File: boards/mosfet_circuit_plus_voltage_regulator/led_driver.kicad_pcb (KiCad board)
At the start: 2 copper layers, 75 x 50 mm, 26 parts, among them J1 Vin, J2 LED, J3 control_in, Q1 IRF4905 P-chan, Q2 BUZ11 N-chan, U1 MC34063AP

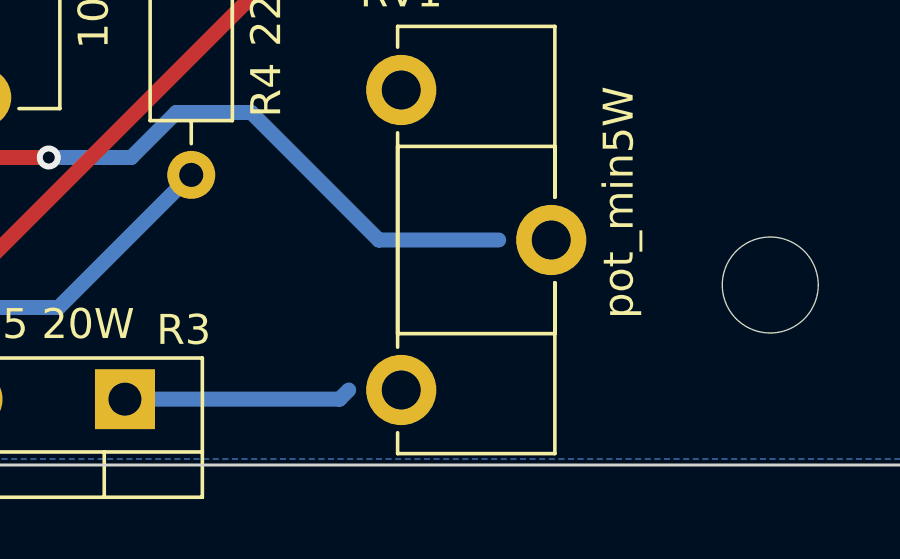
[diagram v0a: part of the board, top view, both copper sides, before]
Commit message: update gerbers
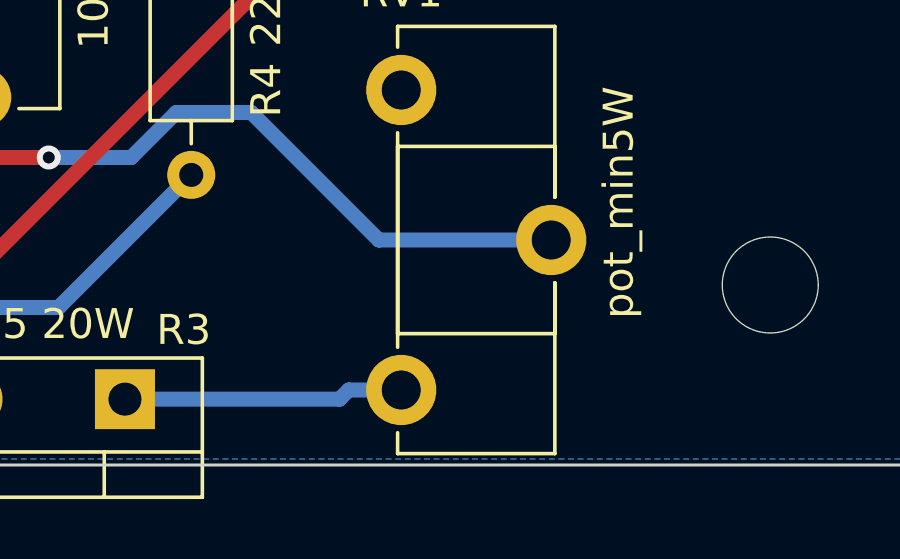
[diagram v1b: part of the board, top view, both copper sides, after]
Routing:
- net Net-(R3-Pad1): track 7.59 -> 9.34 mm
- net Net-(J2-Pad1): track 62.0 -> 63.7 mm
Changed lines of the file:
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@@
   (segment (start 94.485 79.235) (end 108 92.75) (width 0.5) (layer "F.Cu") (net 2))
   (via (at 131.75 92.75) (size 0.8) (drill 0.4) (layers "F.Cu" "B.Cu") (net 2))
-  (segment (start 142.75 95.5) (end 146.75 95.5) (width 0.5) (layer "B.Cu") (net 2))
+  (segment (start 142.75 95.5) (end 148.5 95.5) (width 0.5) (layer "B.Cu") (net 2))
+  (segment (start 136 91.25) (end 138.5 91.25) (width 0.5) (layer "B.Cu") (net 2))
+  (segment (start 131.75 92.75) (end 134.5 92.75) (width 0.5) (layer "B.Cu") (net 2))
   (segment (start 138.5 91.25) (end 142.75 95.5) (width 0.5) (layer "B.Cu") (net 2))
-  (segment (start 131.75 92.75) (end 134.5 92.75) (width 0.5) (layer "B.Cu") (net 2))
   (segment (start 134.5 92.75) (end 136 91.25) (width 0.5) (layer "B.Cu") (net 2))
-  (segment (start 136 91.25) (end 138.5 91.25) (width 0.5) (layer "B.Cu") (net 2))
   (segment (start 139 61) (end 139 80.67) (width 0.5) (layer "F.Cu") (net 3))
   (segment (start 135.25 57.25) (end 139 61) (width 0.5) (layer "F.Cu") (net 3))
@@
   (segment (start 126.8984 78.9808) (end 129.4384 78.9808) (width 0.5) (layer "B.Cu") (net 10))
   (segment (start 129.4384 71.3608) (end 129.4384 78.9808) (width 0.5) (layer "B.Cu") (net 10))
+  (segment (start 141.75 100.5) (end 143.5 100.5) (width 0.5) (layer "B.Cu") (net 11))
   (segment (start 134.29 100.805) (end 141.445 100.805) (width 0.5) (layer "B.Cu") (net 11))
   (segment (start 141.445 100.805) (end 141.75 100.5) (width 0.5) (layer "B.Cu") (net 11))
